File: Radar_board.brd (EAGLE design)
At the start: 160 x 100 mm, 22 parts, among them IC1 555, J1 AUDIO_JACK_3.5MM_PTH, U1 MAX2750AUA+

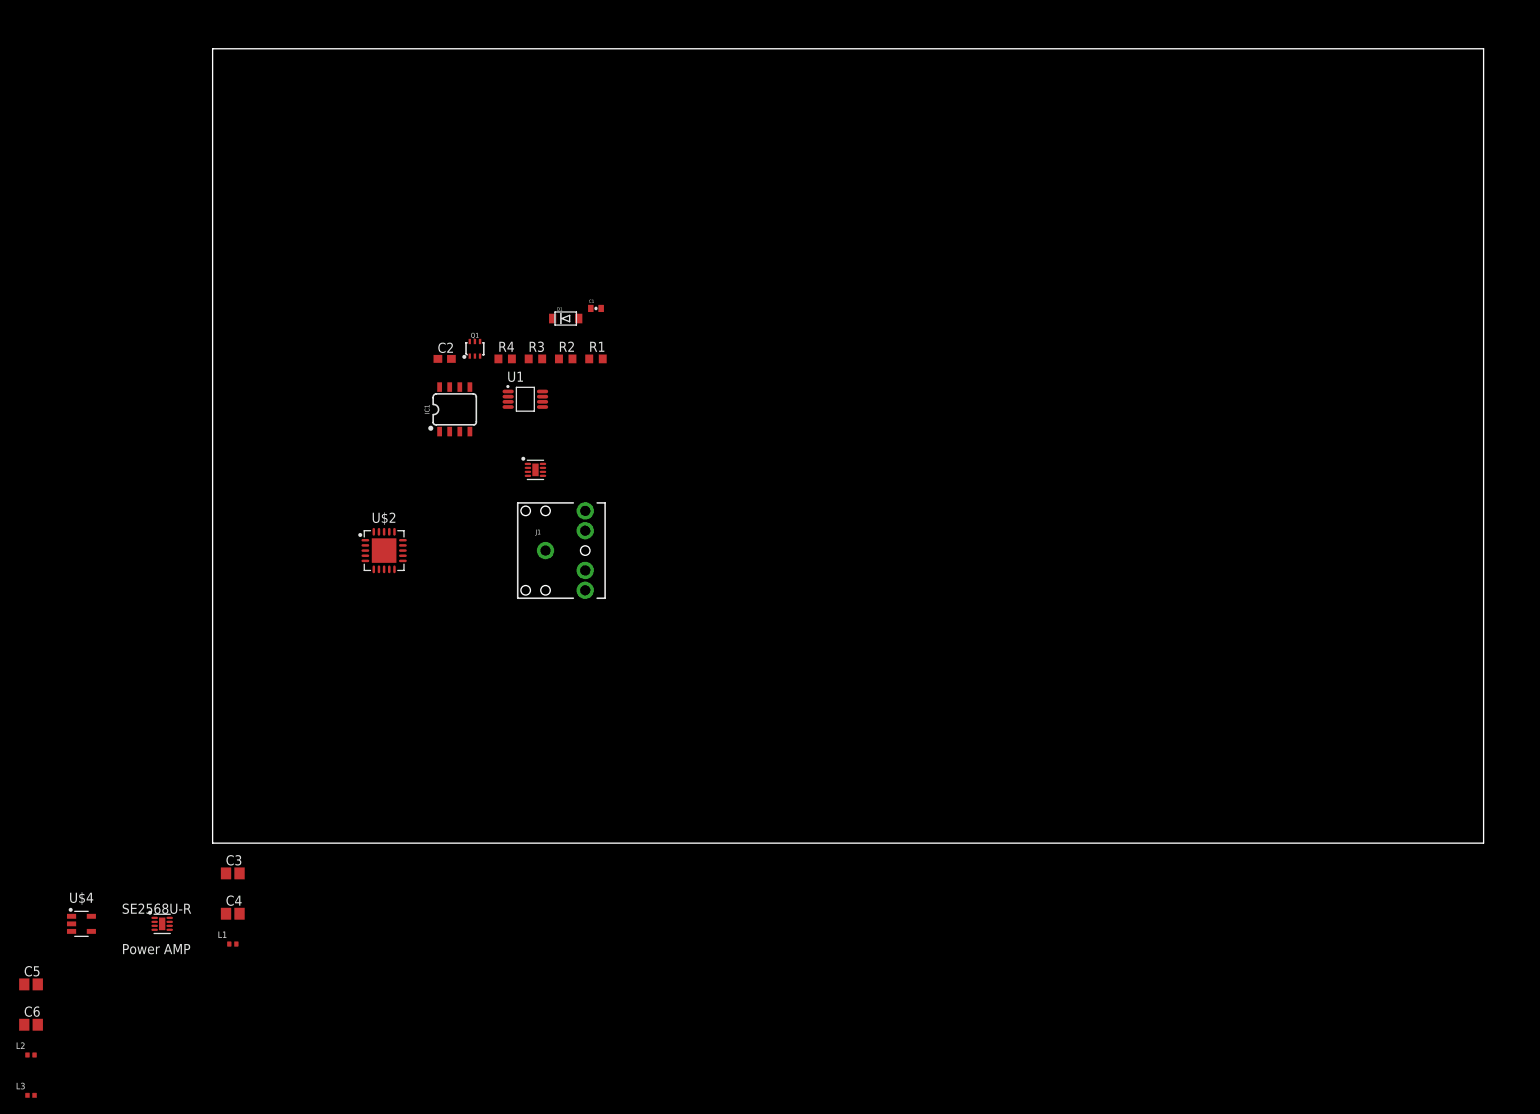
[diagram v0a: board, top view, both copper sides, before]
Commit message: Add files via upload
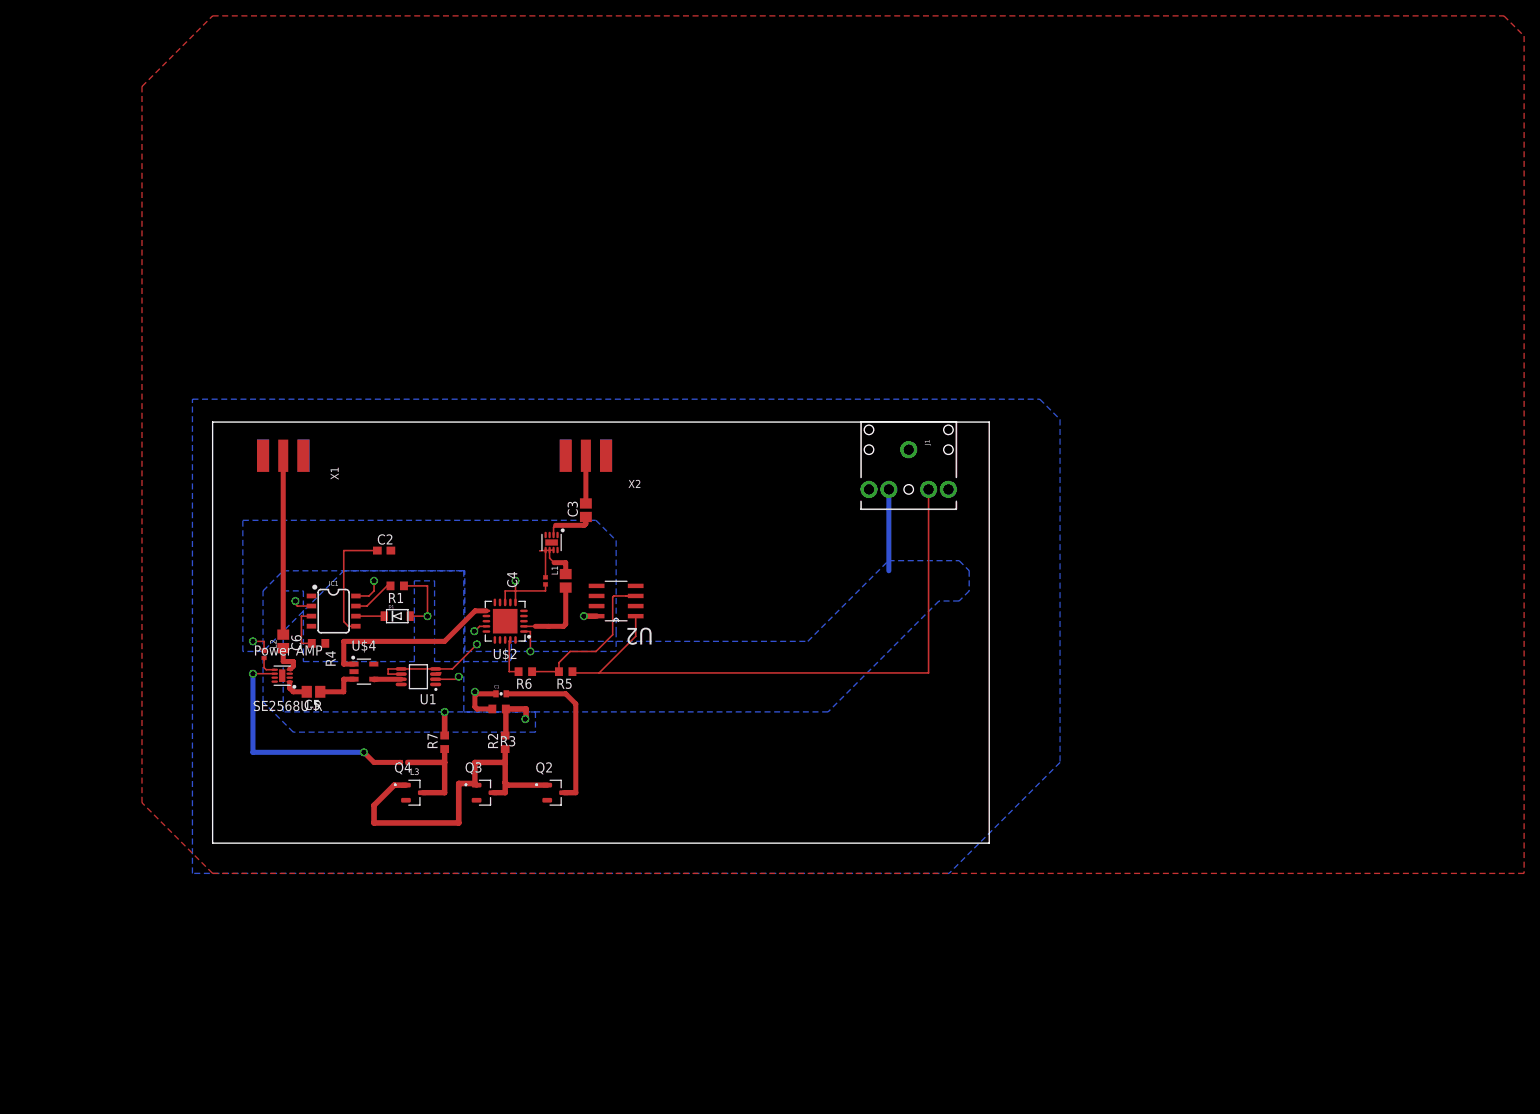
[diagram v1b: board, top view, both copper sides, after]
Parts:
- removed Q1: (no value), SparkFun-DiscreteSemi:SC70-6
- added Q2, Q3, Q4: MMBT2222ALT1, MMBT2222ALT1:SOT95P237X111-3N
- added R5, R6, R7: (no value), adafruit:R0603
- added U2: NE5532DR, NE5532DR:SOIC127P600X175-8N
- added X1, X2: (no value), adafruit:SMA_EDGELAUNCH
- moved C3 63.8 mm to (47.0, 41.9), turned to 90 degrees
- moved L3 63.0 mm to (24.1, 10.2), turned to 180 degrees
- moved L1 60.3 mm to (41.9, 33.0), turned to 270 degrees
- moved C4 59.3 mm to (44.5, 33.0), turned to 90 degrees
- moved L2 58.3 mm to (6.48, 23.7), turned to 270 degrees
- moved C6 57.8 mm to (8.89, 25.4), turned to 270 degrees
- moved C5 51.2 mm to (12.7, 19.1), turned to 180 degrees
- moved C1 50.0 mm to (36.3, 18.8)
- moved R2 48.9 mm to (36.8, 12.7), turned to 90 degrees
- moved U$4 47.7 mm to (19.1, 21.6)
- moved J1 47.5 mm to (87.6, 49.5), turned to 270 degrees
- moved R3 44.3 mm to (36.1, 16.9), turned to 180 degrees
- moved D1 43.1 mm to (23.2, 28.6)
- moved R4 42.8 mm to (13.3, 25.1), turned to 180 degrees
- moved R1 38.0 mm to (23.2, 32.4), turned to 180 degrees
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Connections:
- new net LO_SPLIT: U$2.11, U$4.1
- new net N$14: C6.1, X1.P
- new net N$15: J1.RSH, R5.1, U2.1
- new net N$16: R5.2, R6.1, U2.3
- new net PWRBIAS: L3.1, Q4.3, R7.1
- net 0: now also Q2.2, Q3.2, Q4.2, U2.4, X1.GND@1, X1.GND@2, X1.GND@3, X1.GND@4, X2.GND@1, X2.GND@2, X2.GND@3, X2.GND@4; no longer Q1.1, Q1.4
- net LO: no longer U$2.11, U$4.1
- net N$1: now also Q2.1, Q3.1, Q3.3, Q4.1; no longer Q1.2, Q1.3, Q1.5
- net N$10: now also C3.2, X2.P; no longer C6.1
- net N$11: now also C5.2, U$3.1; no longer L3.1
- net N$13: now also C4.2, U$1.6; no longer L2.1
- net N$2: now also Q2.3; no longer Q1.6
- net N$7: now also L2.2, U$3.5; no longer U$2.1, U$2.8
- net PA_IN: no longer C5.2, U$3.1
- net RFO: no longer C4.2, U$1.6
- net TRIOUT: now also J1.TSH
- net TV_IN: now also R6.2
- net VCC3V: now also R7.2; no longer L2.2, U$3.5
- net VCC6V: now also L2.1, U$2.1, U$2.14, U$2.6, U$2.8, U2.8
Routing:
- net N$15: track 0.00 -> 77.1 mm
- net N$1: track 0.00 -> 44.1 mm
- net VCC6V: track 0.00 -> 34.5 mm, vias 0 -> 6
- net TRIOUT: track 0.00 -> 31.9 mm, vias 0 -> 4
- net VCC1V: track 0.00 -> 31.8 mm, vias 0 -> 2
- net LO_SPLIT: track 0.00 -> 23.7 mm
- net N$14: track 0.00 -> 22.5 mm
- net N$2: track 0.00 -> 21.9 mm
- net N$16: track 0.00 -> 21.7 mm
- net N$5: track 0.00 -> 14.9 mm
- net VCC3V: track 0.00 -> 14.0 mm, vias 0 -> 3
- net PWRBIAS: track 0.00 -> 12.5 mm
- net RFO: track 0.00 -> 10.2 mm
- net N$8: track 0.00 -> 6.06 mm
- net N$4: track 0.00 -> 6.01 mm
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- added copper zone on layer 1, net 0
- added copper zone on layer 16, net GND
- added copper zone on layer 16, net TRIOUT
- added copper zone on layer 16, net VCC3V
- added copper zone on layer 16, net VCC6V
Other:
- board size 160 x 100 mm -> 97.8 x 53 mm
